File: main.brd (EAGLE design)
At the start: 130 x 34 mm, 176 parts, among them CN1 DC-012A-D010, CN2 JST GH 10 Pin, CN3 5.8ZSPT, CN4 8 PIN FFC, CN5 MC-118LS-H100, CN6 JST GH 10 Pin, CN7 8 PIN FFC, Q1 GSFP0449, Q6 IRLML6244, U1 Ti60F225C4, U10 W958D8NBYA5I, U11 TPS70918, U12 AP7335, U2 USBLC6-2SC6, U24 SCHMITT, U25 SCHMITT, U3 93LC56B-I/SN, U4 W25Q128JV, U5 TPS62065, U6 FT2232H, U7 TPS563201, U8 AR0822, U9 TPS62065

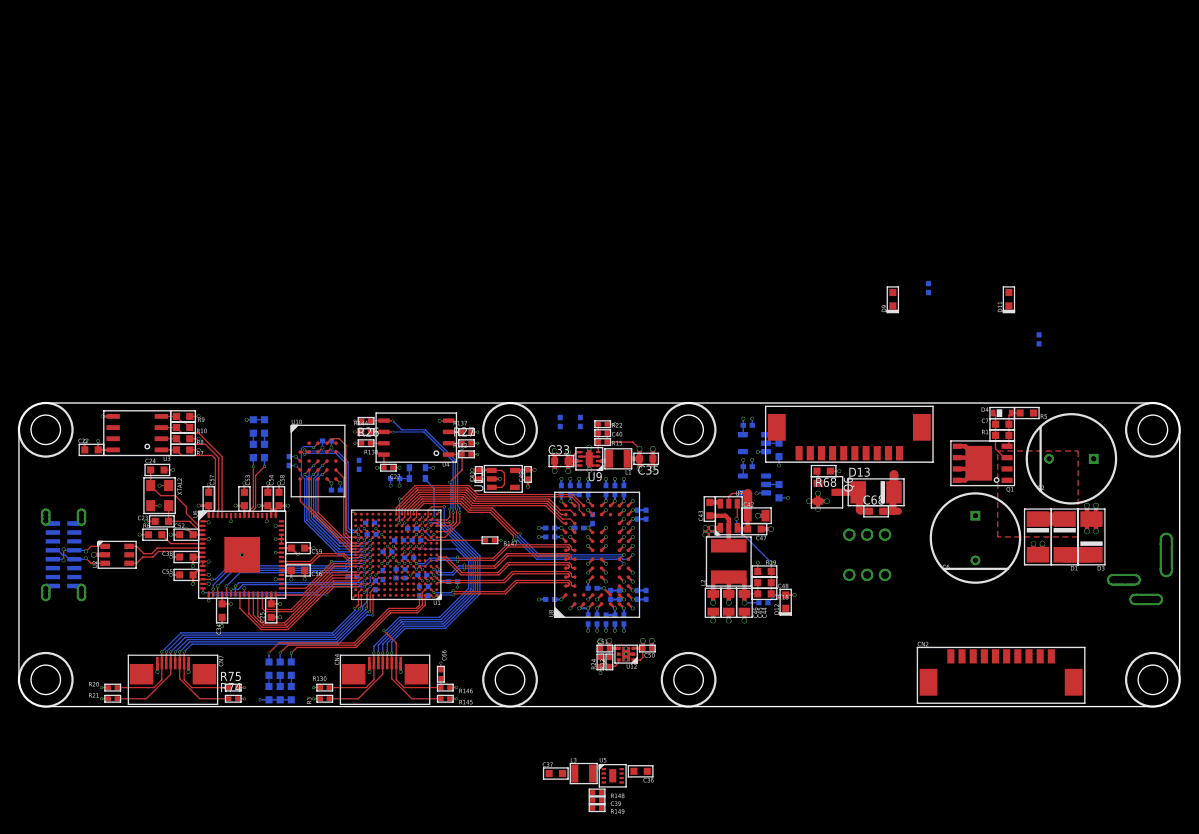
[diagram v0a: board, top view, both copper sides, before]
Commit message: Initial layout done
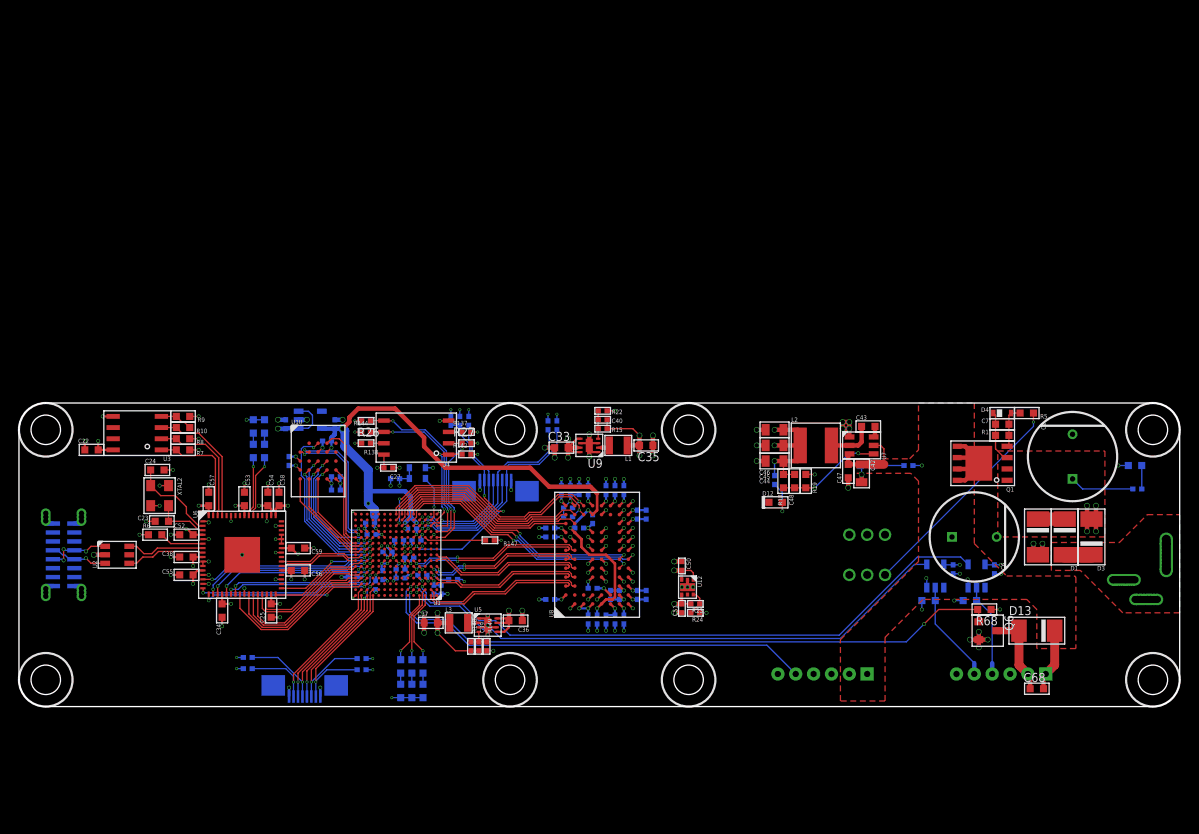
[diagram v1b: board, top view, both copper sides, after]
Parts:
- CN2, CN6: value JST GH 10 Pin -> JST GH 6P V-TH; device CONNECTORs:1.25-10PWT -> CONNECTORs:PH-6P-V-TH
- moved R3 39.5 mm to (-5.75, 14.5), flipped to the bottom, turned to 90 degrees
- moved R130 39.2 mm to (-4.75, 14.5), flipped to the bottom, turned to 90 degrees
- moved CN6 32.3 mm to (45.0, -14.0), flipped to the bottom
- moved C69 32.0 mm to (44.2, -1.62), turned to 90 degrees
- moved R145 31.2 mm to (-14.6, 15.0), flipped to the bottom, turned to 90 degrees
- moved R146 29.9 mm to (-16.6, 15.0), flipped to the bottom, turned to 90 degrees
- moved U24 29.0 mm to (42.2, -2.38), turned to 180 degrees
- moved C66 28.5 mm to (-15.6, 15.0), flipped to the bottom
- moved R72 27.2 mm to (41.5, -5.12), turned to 180 degrees
- moved C68 26.8 mm to (49.0, -15.0)
- moved C70 25.7 mm to (39.6, -1.62), turned to 90 degrees
- moved CN4 23.9 mm to (-11.6, 6.50), flipped to the bottom
- moved D13 23.8 mm to (49.0, -8.50)
- moved Q6 23.8 mm to (43.5, -8.50)
- moved R68 23.8 mm to (43.1, -6.12)
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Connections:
- removed net PWR_FPGA_1V8: C74.2, C77.2, C78.2, C79.2, U1.D4, U1.E11, U1.L4, U1.M11
- removed net TEMP_SEN_A: CN2.2
- removed net TEMP_SEN_B: CN2.1
- net GND: now also CN2.3, CN6.6; no longer CN2.5, CN2.7, CN6.10
- net LED_PWM_CONT: now also CN2.5, U1.C5; no longer CN2.3
- net MTR_CONT_PWM: now also U1.B5
- net MTR_SENSE_A: now also U1.C3
- net MTR_SENSE_B: now also U1.C4
- net MTR_SENSE_IN_A: now also CN6.4; no longer CN6.8
- net MTR_SENSE_IN_B: now also CN6.5; no longer CN6.9
- net N$57: now also CN6.2; no longer CN6.4, CN6.5, CN6.6
- net PWR_BUS_UNREG: now also CN2.1, CN2.2; no longer CN2.10, CN2.8, CN2.9, CN6.2, CN6.3
- net PWR_SYS_1V8: now also C74.2, C77.2, C78.2, C79.2, U1.D4, U1.E11, U1.L4, U1.M11
- net PWR_SYS_3V3: now also CN6.3; no longer CN6.7
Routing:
- net PWR_SYS_1V8: track 28.1 -> 126.2 mm, vias 11 -> 17
- net MTR_CONT_PWM: track 1.43 -> 70.6 mm, vias 0 -> 2
- net MTR_SENSE_A: track 0.00 -> 68.3 mm, vias 0 -> 1
- net MTR_SENSE_B: track 0.00 -> 63.9 mm, vias 0 -> 1
- net LED_PWM_CONT: track 0.00 -> 50.0 mm, vias 0 -> 1
- net GND: track 136.7 -> 161.7 mm, vias 142 -> 156
- net N$11: track 0.00 -> 25.0 mm, vias 0 -> 1
- net PWR_FPGA_0V95: track 5.52 -> 27.0 mm, vias 12 -> 14
- net FPGA_JTAG_TDI: track 29.0 -> 11.7 mm, vias 2 -> 1
- net FPGA_CONF_CSI: track 34.5 -> 17.4 mm, vias 2 -> 1
- net PWR_MIPI_1V2: track 1.54 -> 16.6 mm
- net PROC_UART_RX: track 33.5 -> 19.2 mm, vias 2 -> 1
- net PROC_UART_TX: track 35.2 -> 21.0 mm, vias 2 -> 1
- net PROC_JTAG_TDO: track 34.7 -> 20.7 mm, vias 2 -> 1
- net PROC_JTAG_TCK: track 36.5 -> 22.7 mm, vias 2 -> 3
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- added copper zone on layer 1, net N$5
- added copper zone on layer 1, net PWR_BUS_UNREG
- added copper zone on layer 3, net PWR_FPGA_0V95

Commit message: DRC errors processed
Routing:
- net PWR_SEN_2V8A: track 15.6 -> 18.2 mm
- net PWR_SYS_3V3: track 94.1 -> 95.1 mm
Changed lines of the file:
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@@
 </layers>
 <board>
-<fusionsync huburn="a.YnVzaW5lc3M6bXl1Y2wxNDk2" projecturn="a.YnVzaW5lc3M6bXl1Y2wxNDk2IzIwMjIwMzI1NTEwNjk2MjUx" f3durn="urn:adsk.wipprod:dm.lineage:P9SLlJ01T8W2nK3aE3uNkQ" pcbguid="" lastpulledtime="" lastsyncedchangeguid="" latestrevisionid="3c05b058-9429-4bd3-9ed8-e82aa17abb45" lastsyncedrevisionid="3c05b058-9429-4bd3-9ed8-e82aa17abb45" lastboardhashguid="c5c7c101-7b9a-4bde-de48-64a6e5410f6e" lastpushedtime="2024-03-16T13:46:00Z" linktopcb3d="true"/>
+<fusionsync huburn="a.YnVzaW5lc3M6bXl1Y2wxNDk2" projecturn="a.YnVzaW5lc3M6bXl1Y2wxNDk2IzIwMjIwMzI1NTEwNjk2MjUx" f3durn="urn:adsk.wipprod:dm.lineage:P9SLlJ01T8W2nK3aE3uNkQ" pcbguid="" lastpulledtime="" lastsyncedchangeguid="" latestrevisionid="090a522b-cd39-4de5-9746-b6cb41953c83" lastsyncedrevisionid="090a522b-cd39-4de5-9746-b6cb41953c83" lastboardhashguid="c91166a2-c907-744a-d8fd-3564c5b6663c" lastpushedtime="2024-03-16T15:48:05Z" linktopcb3d="true"/>
 <plain>
 <wire x1="-65" y1="14" x2="-65" y2="-14" width="0" layer="20" locked="yes"/>
@@
 <wire x1="-35.125" y1="14.125" x2="-35.075" y2="14.175" width="0.5" layer="16"/>
 <wire x1="-35.075" y1="14.175" x2="-33.625" y2="14.175" width="0.5" layer="16"/>
-<wire x1="-20.15" y1="0.65" x2="-20.15" y2="-3.9" width="0" layer="19" extent="1-1"/>
+<wire x1="-20.45" y1="-4.2" x2="-19.55" y2="-4.2" width="0.3" layer="3"/>
+<wire x1="-19.55" y1="-4.2" x2="-19.5" y2="-4.25" width="0.3" layer="3"/>
 </signal>
 <signal name="PWR_FPGA_0V95">
@@
 <contactref element="U6" pad="54"/>
 <contactref element="D8" pad="K"/>
-<wire x1="-37.5" y1="10.875" x2="-37.25" y2="11.125" width="0.15" layer="16"/>
 <wire x1="-38.75" y1="4.4" x2="-38.75" y2="5" width="0.1016" layer="1"/>
 <wire x1="-38.75" y1="5" x2="-38.5" y2="5.25" width="0.1016" layer="1"/>
@@
 <contactref element="D13" pad="K"/>
 <contactref element="C68" pad="2"/>
-<wire x1="50.875" y1="-8.625" x2="51" y2="-8.5" width="0.8" layer="1"/>
 <contactref element="CN6" pad="1"/>
 <contactref element="CN2" pad="1"/>
@@
 <contactref element="D13" pad="A"/>
 <contactref element="Q6" pad="2"/>
-<wire x1="47" y1="-8.5" x2="47.125" y2="-8.625" width="0.8" layer="1"/>
 <contactref element="C68" pad="1"/>
 <wire x1="44.5" y1="-8.5" x2="47" y2="-8.5" width="0.8" layer="1"/>
@@
 <wire x1="9.25" y1="-5.5" x2="10.25" y2="-5.5" width="0.15" layer="1"/>
 <polygon width="0.15" layer="3" rank="2">
-<vertex x="-5" y="-3.625"/>
-<vertex x="9.5" y="-3.625"/>
+<vertex x="-5" y="7"/>
+<vertex x="7.125" y="7"/>
+<vertex x="7.125" y="-4.625"/>
+<vertex x="9.5" y="-4.625"/>
 <vertex x="9.5" y="-10.5"/>
 <vertex x="-5" y="-10.5"/>
 </polygon>
-<wire x1="3.75" y1="5" x2="3.25" y2="5.5" width="0" layer="19" extent="1-1"/>
-<wire x1="1.75" y1="6" x2="3.25" y2="5.5" width="0" layer="19" extent="1-1"/>
-<wire x1="3.25" y1="-4.5" x2="3.25" y2="4.5" width="0" layer="19" extent="1-1"/>
+<wire x1="1.75" y1="6" x2="2.25" y2="5.5" width="0.3" layer="3"/>
+<wire x1="2.25" y1="5.5" x2="3.5" y2="5.5" width="0.3" layer="3"/>
+<wire x1="3.5" y1="5.5" x2="3.75" y2="5.75" width="0.3" layer="3"/>
+<wire x1="3.75" y1="5.75" x2="3.75" y2="6" width="0.3" layer="3"/>
 </signal>
 <signal name="PWR_SYS_1V8">
@@
 <vertex x="3.75" y="14"/>
 <vertex x="5.125" y="14"/>
-<vertex x="5.125" y="1.125"/>
-<vertex x="3.25" y="1.125"/>
+<vertex x="5.125" y="6.75"/>
+<vertex x="3.25" y="6.75"/>
 <vertex x="3.25" y="-5.5"/>
 <vertex x="2.25" y="-5.5"/>
@@
 <contactref element="C76" pad="2"/>
 <contactref element="C75" pad="2"/>
-<wire x1="-18.975" y1="-2.475" x2="-18.525" y2="-2.925" width="0.3" layer="3"/>
-<wire x1="-19.825" y1="-1.625" x2="-19.04645" y2="-2.40355" width="0.5" layer="3"/>
+<wire x1="-18.525" y1="-2.925" x2="-19.1" y2="-2.35" width="0.3" layer="3"/>
+<wire x1="-19.825" y1="-1.625" x2="-19.1" y2="-2.35" width="0.5" layer="3"/>
 <wire x1="-18.525" y1="-2.925" x2="-15.2" y2="-2.925" width="0.5" layer="3"/>
 <wire x1="-15.2" y1="-2.925" x2="-15.125" y2="-3" width="0.5" layer="3"/>
@@
 <wire x1="-18.525" y1="-3.4" x2="-18.525" y2="-2.925" width="0.25" layer="16"/>
 <wire x1="-18.525" y1="-3.4" x2="-17.7125" y2="-3.4" width="0.25" layer="16"/>
-<wire x1="-18.975" y1="-2.475" x2="-19.04645" y2="-2.40355" width="0" layer="19" extent="3-3"/>
 </signal>
 <signal name="RAM_NRESET">
@@
 <mfgpreviewcolors>
 <mfgpreviewcolor name="soldermaskcolor" color="0xC80C0C0C"/>
-<mfgpreviewcolor name="silkscreencolor" color="0xFF0C0C0C"/>
+<mfgpreviewcolor name="silkscreencolor" color="0xFFDEDEDE"/>
 <mfgpreviewcolor name="backgroundcolor" color="0xFF282828"/>
 <mfgpreviewcolor name="coppercolor" color="0xFFD3D3D3"/>
 <mfgpreviewcolor name="substratecolor" color="0xFF181818"/>
 </mfgpreviewcolors>
+<errors>
+</errors>
 </board>
 </drawing>

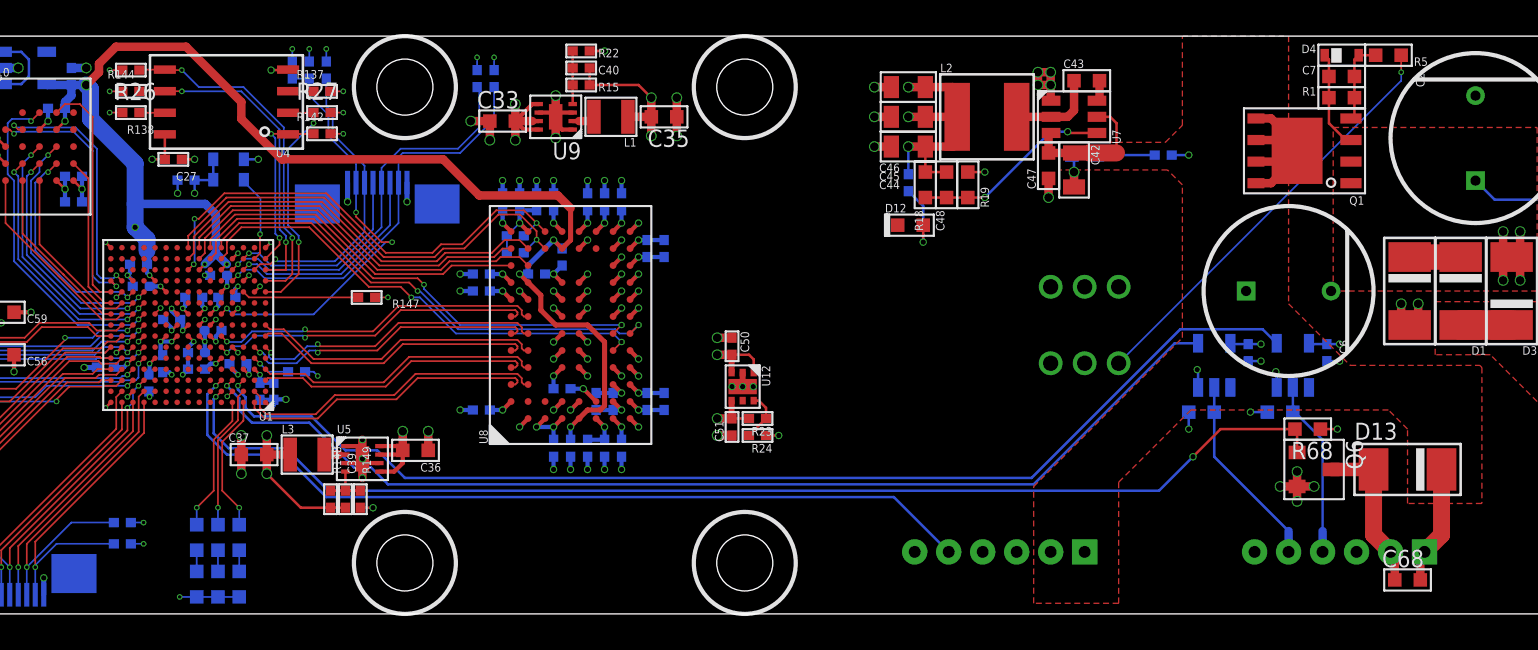
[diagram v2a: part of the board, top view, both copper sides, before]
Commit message: New LED driver PCB
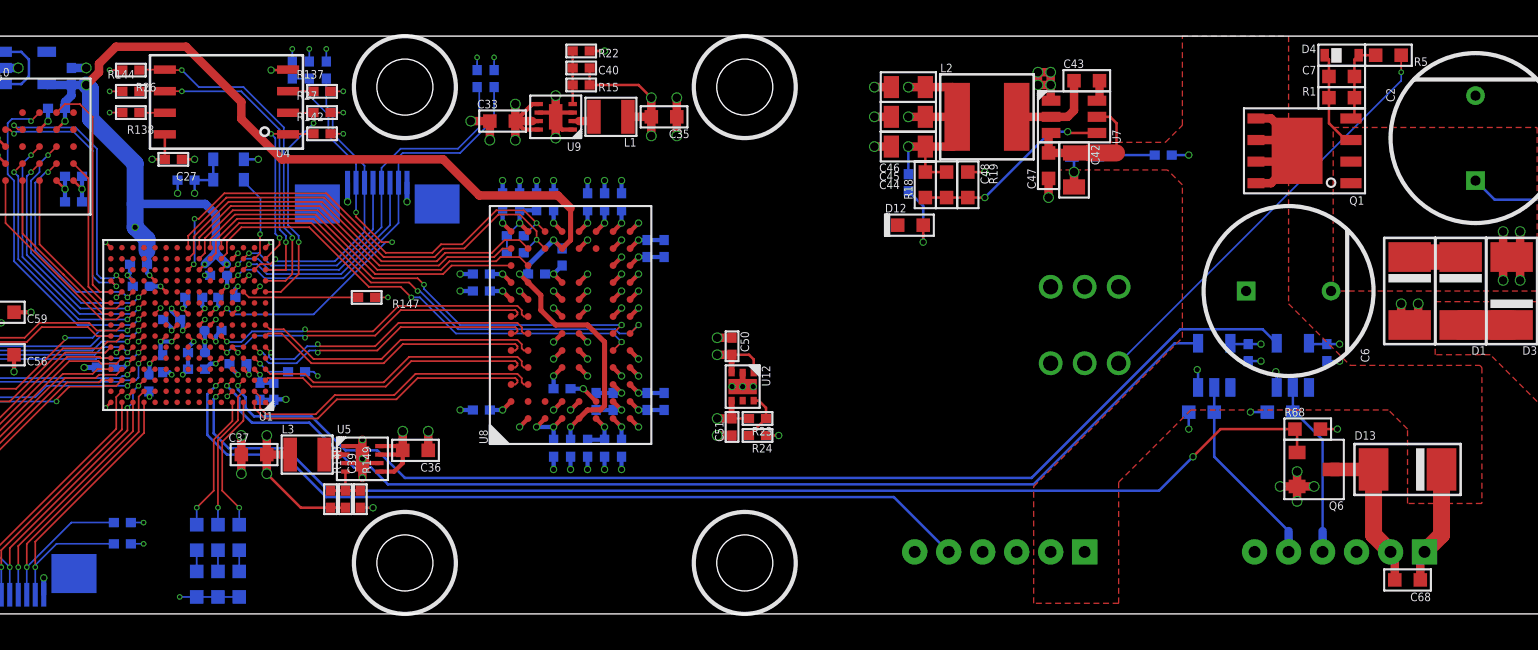
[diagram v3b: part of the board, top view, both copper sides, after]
